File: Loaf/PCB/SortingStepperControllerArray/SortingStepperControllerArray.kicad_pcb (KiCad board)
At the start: 2 copper layers, 100 x 73 mm, 26 parts, among them J1 Conn_01x04_Socket, J2 Conn_01x04_Socket, J3 Conn_01x04_Socket, J4 Conn_01x04_Socket, J5 Motor_Supply, J6 Logic_Supply, J7 Logic_Input, SW1 Limit_Switch, SW2 Limit_Switch, SW3 Limit_Switch, SW4 Limit_Switch

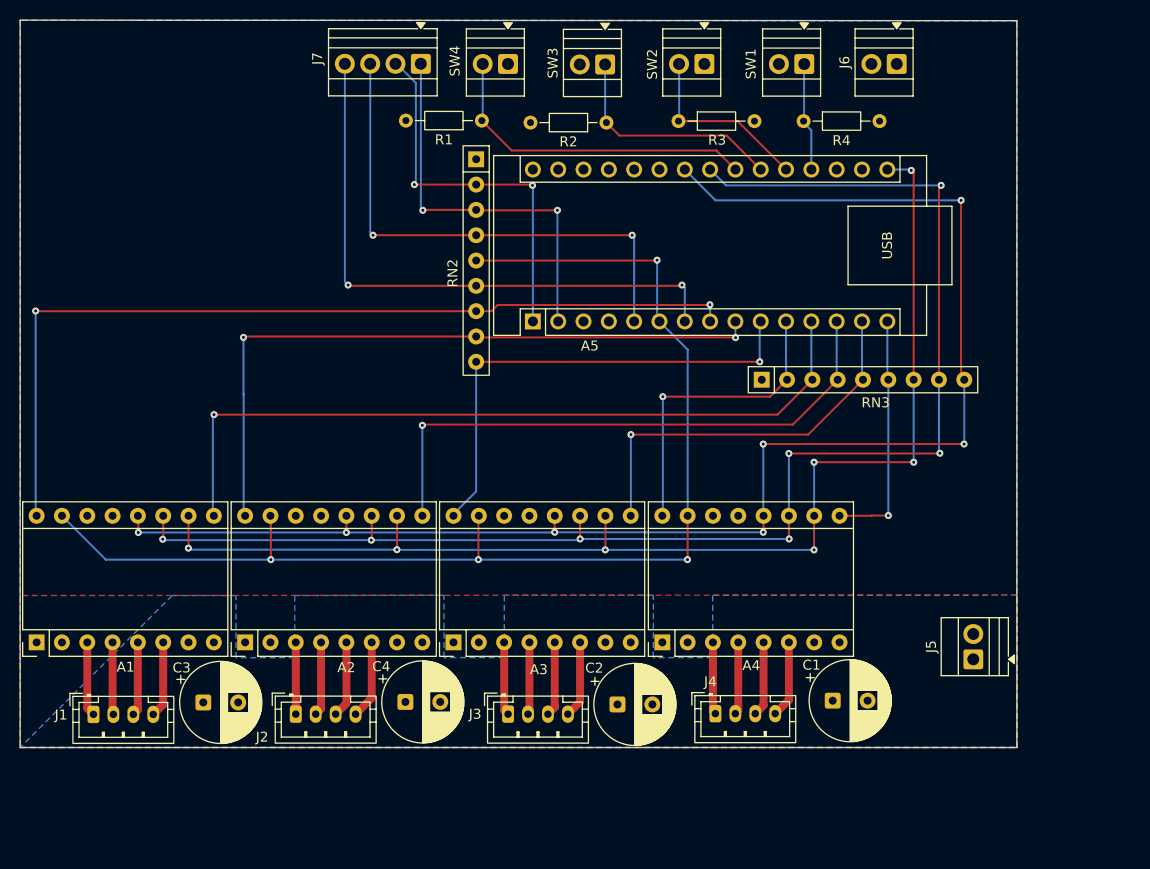
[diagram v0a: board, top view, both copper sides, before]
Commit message: Redid the stepper board
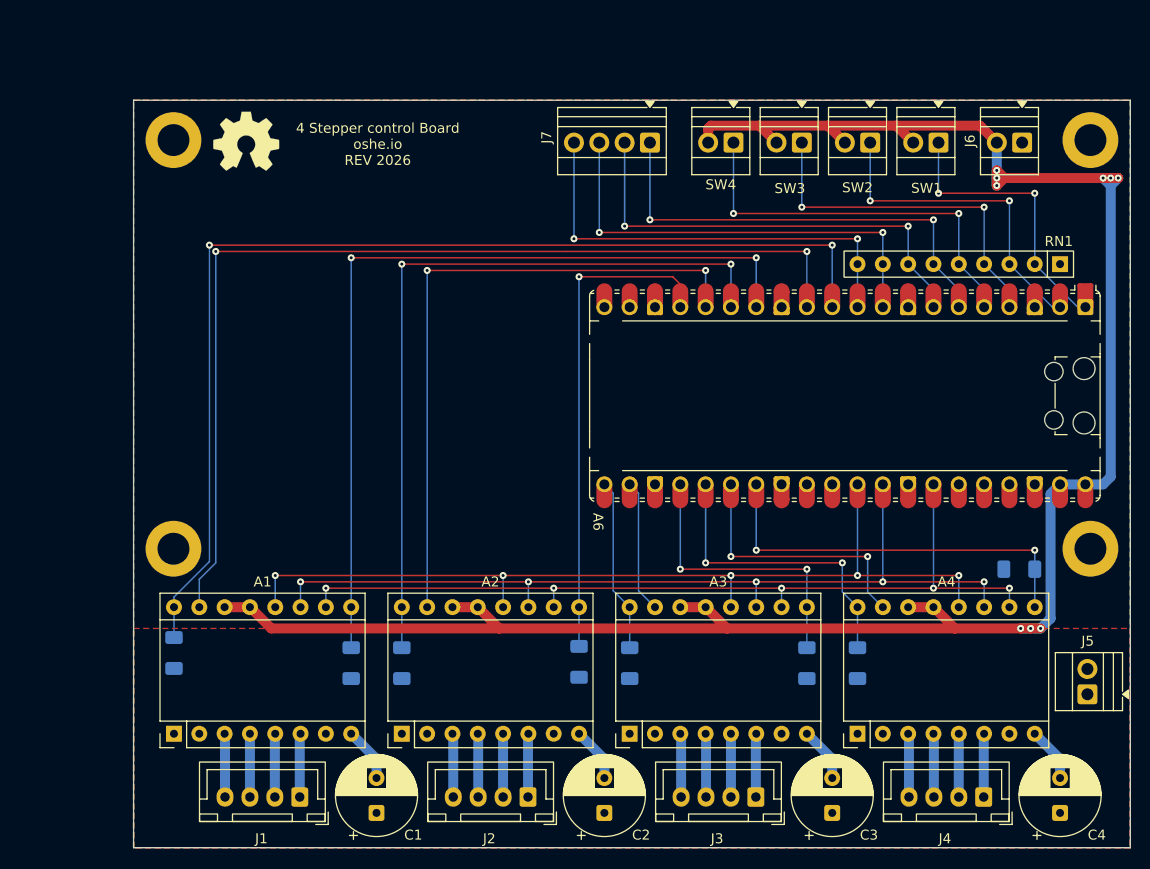
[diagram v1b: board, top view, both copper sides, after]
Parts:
- removed A5: Arduino_Nano_Every, Module:Arduino_Nano
- removed RN2, RN3: 10K Resistor Array, Resistor_THT:R_Array_SIP9
- added A6: RaspberryPi_Pico, Module:RaspberryPi_Pico_Common_Unspecified, F.Cu at (180.3, 94.1)
- added H1: MountingHole_Pad, MountingHole:MountingHole_3.2mm_M3_DIN965_Pad, F.Cu at (113.0, 68.5)
- added H2: MountingHole_Pad, MountingHole:MountingHole_3.2mm_M3_DIN965_Pad, F.Cu at (205.0, 68.5)
- added H3: MountingHole_Pad, MountingHole:MountingHole_3.2mm_M3_DIN965_Pad, F.Cu at (113.0, 109.5)
- added H4: MountingHole_Pad, MountingHole:MountingHole_3.2mm_M3_DIN965_Pad, F.Cu at (205.0, 109.5)
- added Logo1: Logo_Open_Hardware_Small, Symbol:OSHW-Symbol_6.7x6mm_SilkScreen, F.Cu at (120.3, 68.6)
- added R5: 10K, Resistor_SMD:R_1206_3216Metric_Pad1.30x1.75mm_HandSolder, B.Cu at (176.5, 120.9)
- added R6: 10K, Resistor_SMD:R_1206_3216Metric_Pad1.30x1.75mm_HandSolder, B.Cu at (158.8, 120.9)
- added R7: 10K, Resistor_SMD:R_1206_3216Metric_Pad1.30x1.75mm_HandSolder, B.Cu at (197.8, 111.5)
- added R8: 10K, Resistor_SMD:R_1206_3216Metric_Pad1.30x1.75mm_HandSolder, B.Cu at (181.6, 120.9)
- added RN1: 10K Resistor Array, Resistor_THT:R_Array_SIP9, F.Cu at (201.9, 80.9)
- J1, J2, J3, J4: footprint Connector_JST:JST_PH_B4B-PH-K_1x04_P2.00mm_Vertical -> Connector_JST:JST_XH_B4B-XH-A_1x04_P2.50mm_Vertical
- R1, R2, R3, R4: footprint Resistor_THT:R_Axial_DIN0204_L3.6mm_D1.6mm_P7.62mm_Horizontal -> Resistor_SMD:R_1206_3216Metric_Pad1.30x1.75mm_HandSolder; moved to B.Cu
- moved R2 68.7 mm to (113.0, 119.9), turned to 90 degrees
- moved R4 67.7 mm to (135.9, 120.9), turned to 90 degrees
- moved C4 66.6 mm to (201.9, 136.0), turned to 90 degrees
- moved C3 64.1 mm to (179.1, 136.0), turned to 90 degrees
- moved R1 56.0 mm to (130.8, 120.9), turned to 90 degrees
- moved R3 55.2 mm to (153.7, 120.8), turned to 90 degrees
- moved C1 47.1 mm to (133.3, 136.0), turned to 90 degrees
- moved J4 28.2 mm to (194.3, 134.4), turned to 180 degrees
- moved J3 26.2 mm to (171.4, 134.4), turned to 180 degrees
- moved J2 24.7 mm to (148.6, 134.4), turned to 180 degrees
- moved J7 24.3 mm to (160.8, 68.7)
- moved SW4 24.0 mm to (169.2, 68.7)
- moved J1 22.3 mm to (125.7, 134.4), turned to 180 degrees
- moved A4 21.6 mm to (181.6, 128.0)
- moved SW3 21.2 mm to (176.0, 68.7)
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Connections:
- A1 pad 1: GND2 -> GND
- A1 pad 15: /STEP -> /Step1
- A1 pad 2: GND2 -> GND
- A1 pad 7: GND1 -> GND
- A2 pad 1: GND2 -> GND
- A2 pad 15: /STEP -> /Step2
- A2 pad 2: GND2 -> GND
- A2 pad 7: GND1 -> GND
- A3 pad 1: GND2 -> GND
- A3 pad 15: /STEP -> /Step3
- A3 pad 2: GND2 -> GND
- A3 pad 7: GND1 -> GND
- A4 pad 1: GND2 -> GND
- A4 pad 15: /STEP -> /Step4
- A4 pad 2: GND2 -> GND
- A4 pad 7: GND1 -> GND
- C1 pad 1: GND1 -> GND
- C2 pad 1: GND1 -> GND
- C3 pad 1: GND1 -> GND
- C4 pad 1: GND1 -> GND
- J1 pad 1: Net-(A1-A2) -> Net-(A1-B2)
- J1 pad 2: Net-(A1-A1) -> Net-(A1-B1)
- J1 pad 3: Net-(A1-B1) -> Net-(A1-A1)
- J1 pad 4: Net-(A1-B2) -> Net-(A1-A2)
- J2 pad 1: Net-(A2-A2) -> Net-(A2-B2)
- J2 pad 2: Net-(A2-A1) -> Net-(A2-B1)
- J2 pad 3: Net-(A2-B1) -> Net-(A2-A1)
- J2 pad 4: Net-(A2-B2) -> Net-(A2-A2)
- J3 pad 1: Net-(A3-A2) -> Net-(A3-B2)
- J3 pad 2: Net-(A3-A1) -> Net-(A3-B1)
- J3 pad 3: Net-(A3-B1) -> Net-(A3-A1)
- J3 pad 4: Net-(A3-B2) -> Net-(A3-A2)
- J4 pad 1: Net-(A4-A2) -> Net-(A4-B2)
- J4 pad 2: Net-(A4-A1) -> Net-(A4-B1)
- J4 pad 3: Net-(A4-B1) -> Net-(A4-A1)
- J4 pad 4: Net-(A4-B2) -> Net-(A4-A2)
- J5 pad 1: GND1 -> VMOT
- J5 pad 2: VMOT -> GND
- J6 pad 1: GND2 -> GND
- R1 pad 1: /Limit_4 -> GND
- R1 pad 2: GND2 -> /Motor_1_EN
- R2 pad 1: /Limit_3 -> GND
- R2 pad 2: GND2 -> /Motor_1_DIR
- R3 pad 1: /Limit_2 -> GND
- R3 pad 2: GND2 -> /Motor_2_EN
- R4 pad 1: /Limit_1 -> GND
- R4 pad 2: GND2 -> /Motor_2_DIR
- SW2 pad 1: +5V -> /Limit_2
- SW2 pad 2: /Limit_2 -> +5V
- SW4 pad 1: +5V -> /Limit_4
- SW4 pad 2: /Limit_4 -> +5V
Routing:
- net +5V: track 0.00 -> 218.5 mm, vias 0 -> 9
- net /STEP: track 122.9 -> 0.00 mm, vias 4 -> 0
- net /Step1: track 0.00 -> 101.3 mm, vias 0 -> 2
- net /Step2: track 0.00 -> 65.4 mm, vias 0 -> 2
- net /MODE_2: track 150.4 -> 90.4 mm, vias 7 -> 5
- net /MODE_1: track 144.7 -> 88.5 mm, vias 7 -> 5
- net /MODE_0: track 123.6 -> 86.6 mm, vias 7 -> 5
- net /Motor_3_DIR: track 49.0 -> 17.4 mm, vias 1 -> 0
- net /Step4: track 0.00 -> 26.7 mm, vias 0 -> 2
- net VMOT: track 0.00 -> 22.0 mm
- net /Motor_1_DIR: track 90.2 -> 109.5 mm
- net /Limit_1: track 11.1 -> 28.7 mm, vias 0 -> 2
- net /Motor_4_EN: track 24.7 -> 40.3 mm, vias 1 -> 2
- net /Motor_4: track 59.8 -> 45.0 mm
- net /Limit_2: track 18.7 -> 33.0 mm, vias 0 -> 2
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- added copper zone on B.Cu, net GND
- added copper zone on F.Cu, net GND
- removed copper zone on F.Cu, net +5V
- removed copper zone on B.Cu, net GND1
- removed copper zone on B.Cu, net GND2
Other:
- board size 100 x 73 mm -> 100 x 75 mm
- board text added: "4 Stepper control Board oshe.io REV 2026"
